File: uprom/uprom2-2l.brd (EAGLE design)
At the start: 40.6 x 25.4 mm, 7 parts, among them IC1 27C128P, IC2 74AC00D

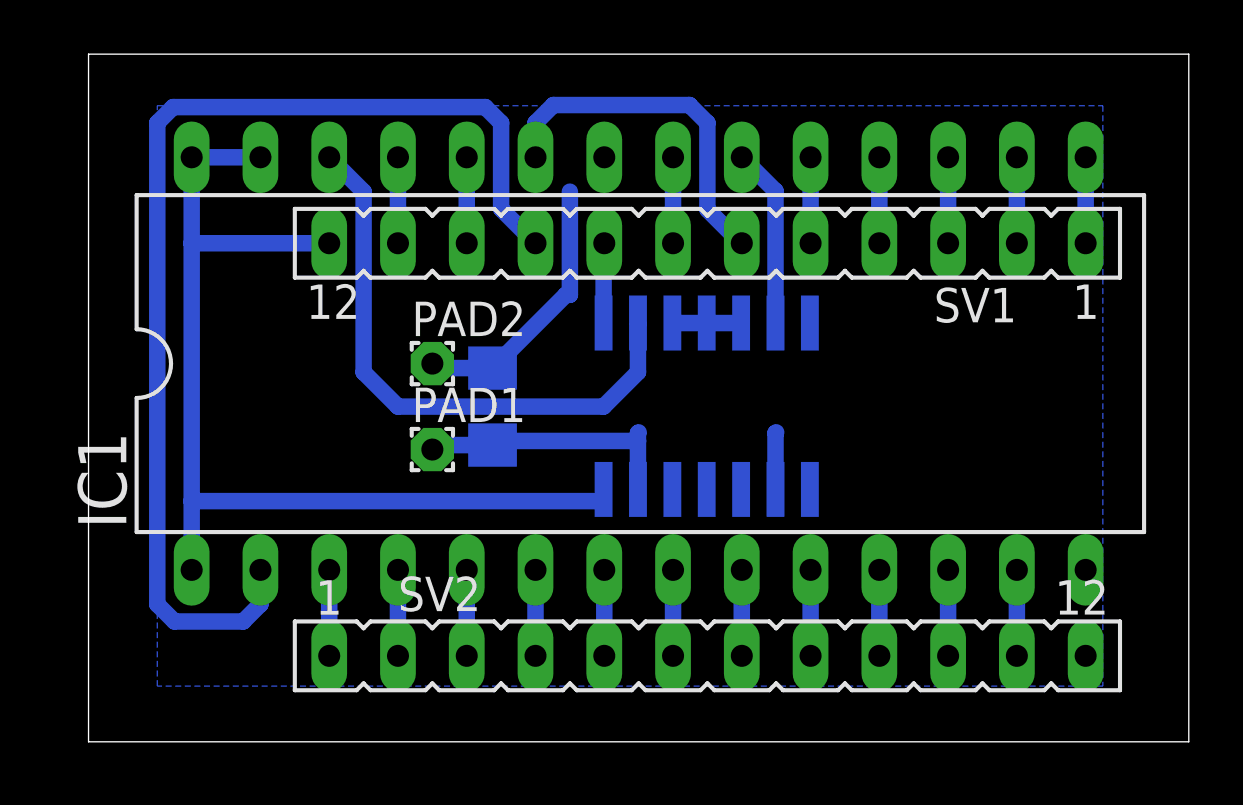
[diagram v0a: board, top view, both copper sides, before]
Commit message: final boards
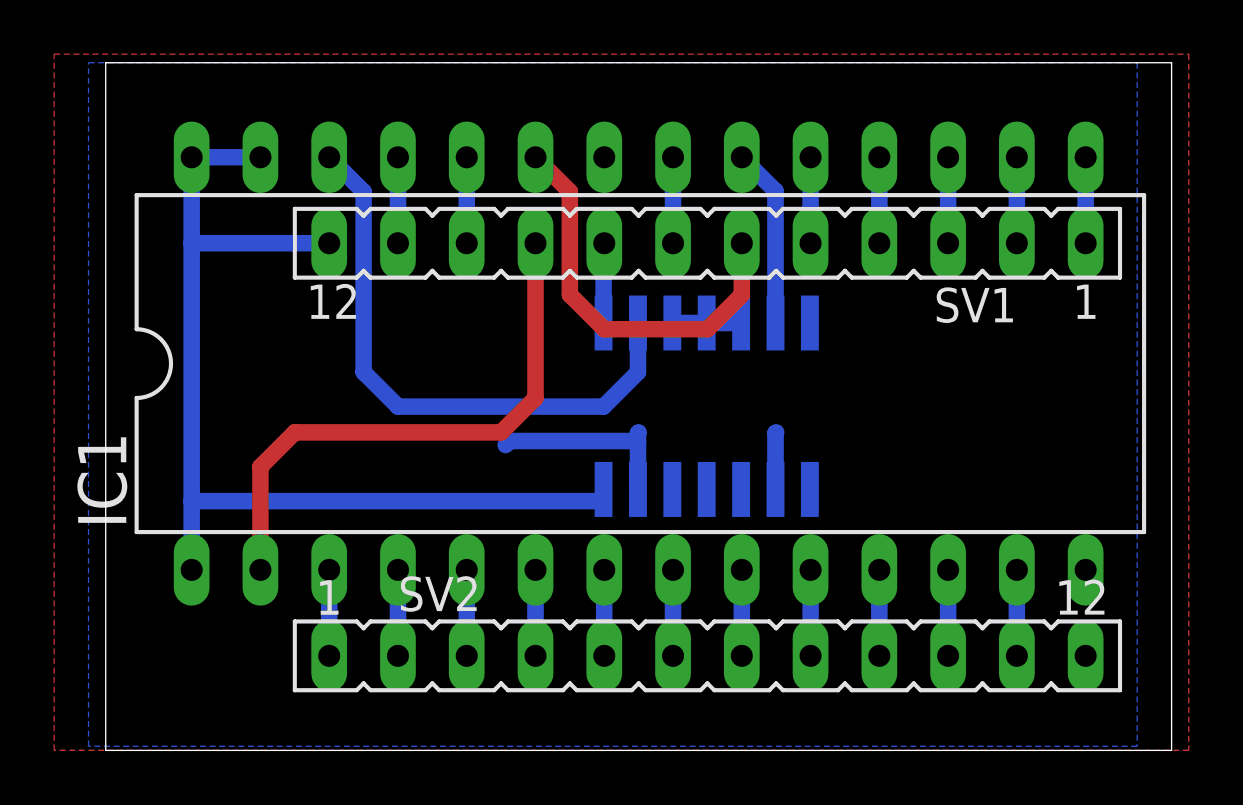
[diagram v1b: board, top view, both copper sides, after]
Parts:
- removed PAD1, PAD2: (no value), wirepad:1,6/0,8
- removed R1: (no value), rcl:R1206
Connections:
- net GND: no longer PAD1.1, PAD2.1, R1.1, R1.2
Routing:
- net A12: track 41.5 -> 20.7 mm
- net GND: track 22.0 -> 9.19 mm
- net A11: track 13.2 -> 14.9 mm
- added copper zone on layer 1, net GND
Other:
- board size 40.6 x 25.4 mm -> 39.4 x 25.4 mm
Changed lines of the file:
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@@
 <board>
 <plain>
-<wire x1="-62.23" y1="73.66" x2="-21.59" y2="73.66" width="0" layer="20"/>
-<wire x1="-21.59" y1="73.66" x2="-21.59" y2="99.06" width="0" layer="20"/>
-<wire x1="-21.59" y1="99.06" x2="-62.23" y2="99.06" width="0" layer="20"/>
-<wire x1="-62.23" y1="99.06" x2="-62.23" y2="73.66" width="0" layer="20"/>
+<wire x1="-61.595" y1="73.3425" x2="-22.225" y2="73.3425" width="0" layer="20"/>
+<wire x1="-22.225" y1="73.3425" x2="-22.225" y2="98.7425" width="0" layer="20"/>
+<wire x1="-22.225" y1="98.7425" x2="-61.595" y2="98.7425" width="0" layer="20"/>
+<wire x1="-61.595" y1="98.7425" x2="-61.595" y2="73.3425" width="0" layer="20"/>
 </plain>
 <attributes>
@@
 <attribute name="VALUE" x="-42.5704" y="86.8172" size="1.27" layer="28" ratio="10" rot="MR180"/>
 </element>
-<element name="R1" library="rcl" library_urn="urn:adsk.eagle:library:334" package="R1206" package3d_urn="urn:adsk.eagle:package:23540/2" value="" x="-47.3075" y="86.0425" smashed="yes" rot="MR270">
-<attribute name="NAME" x="-48.5775" y="87.3125" size="1.27" layer="26" rot="MR270"/>
-<attribute name="POPULARITY" value="41" x="-47.3075" y="86.0425" size="1.778" layer="28" rot="MR270" display="off"/>
-<attribute name="SPICEPREFIX" value="R" x="-47.3075" y="86.0425" size="1.778" layer="28" rot="MR270" display="off"/>
-<attribute name="VALUE" x="-44.7675" y="87.3125" size="1.27" layer="28" rot="MR270"/>
-</element>
-<element name="PAD1" library="wirepad" library_urn="urn:adsk.eagle:library:412" package="1,6/0,8" package3d_urn="urn:adsk.eagle:package:30830/1" value="" x="-49.53" y="84.455" smashed="yes">
-<attribute name="NAME" x="-50.292" y="85.471" size="1.27" layer="25" ratio="10"/>
-<attribute name="POPULARITY" value="15" x="-49.53" y="84.455" size="1.778" layer="27" display="off"/>
-<attribute name="VALUE" x="-49.53" y="85.055" size="0.0254" layer="27"/>
-</element>
-<element name="PAD2" library="wirepad" library_urn="urn:adsk.eagle:library:412" package="1,6/0,8" package3d_urn="urn:adsk.eagle:package:30830/1" value="" x="-49.53" y="87.63" smashed="yes">
-<attribute name="NAME" x="-50.292" y="88.646" size="1.27" layer="25" ratio="10"/>
-<attribute name="POPULARITY" value="15" x="-49.53" y="87.63" size="1.778" layer="27" display="off"/>
-<attribute name="VALUE" x="-49.53" y="88.23" size="0.0254" layer="27"/>
-</element>
 </elements>
 <signals>
@@
 <contactref element="IC1" pad="14"/>
 <contactref element="SV2" pad="12"/>
-<polygon width="0.508" layer="16" isolate="0.4064">
-<vertex x="-59.69" y="75.7174"/>
-<vertex x="-59.69" y="97.155"/>
-<vertex x="-24.765" y="97.155"/>
-<vertex x="-24.765" y="75.7174"/>
+<polygon width="0.508" layer="16" isolate="0.8128">
+<vertex x="-62.23" y="73.4949"/>
+<vertex x="-62.23" y="98.7425"/>
+<vertex x="-23.495" y="98.7425"/>
+<vertex x="-23.495" y="73.4949"/>
 </polygon>
 <contactref element="IC2" pad="7"/>
@@
 <wire x1="-36.8554" y1="85.0646" x2="-36.83" y2="85.09" width="0.6096" layer="16"/>
 <contactref element="IC1" pad="22"/>
-<contactref element="R1" pad="1"/>
-<contactref element="R1" pad="2"/>
-<wire x1="-47.3075" y1="84.6205" x2="-46.8245" y2="84.6205" width="0.6096" layer="16"/>
 <wire x1="-46.8245" y1="84.6205" x2="-46.6725" y2="84.7725" width="0.6096" layer="16"/>
 <wire x1="-46.6725" y1="84.7725" x2="-41.9354" y2="84.7725" width="0.6096" layer="16"/>
-<wire x1="-47.3075" y1="87.4645" x2="-44.602" y2="90.17" width="0.6096" layer="16"/>
-<wire x1="-44.602" y1="90.17" x2="-44.45" y2="90.17" width="0.6096" layer="16"/>
-<wire x1="-44.45" y1="90.17" x2="-44.45" y2="93.98" width="0.6096" layer="16"/>
-<contactref element="PAD1" pad="1"/>
-<contactref element="PAD2" pad="1"/>
-<wire x1="-47.3075" y1="87.4645" x2="-49.3645" y2="87.4645" width="0.6096" layer="16"/>
-<wire x1="-49.3645" y1="87.4645" x2="-49.53" y2="87.63" width="0.6096" layer="16"/>
-<wire x1="-47.3075" y1="84.6205" x2="-49.3645" y2="84.6205" width="0.6096" layer="16"/>
-<wire x1="-49.3645" y1="84.6205" x2="-49.53" y2="84.455" width="0.6096" layer="16"/>
-<wire x1="-47.3075" y1="84.6205" x2="-47.3075" y2="87.4645" width="0" layer="19" extent="16-16"/>
+<polygon width="0.6096" layer="1" isolate="0.4064">
+<vertex x="-63.5" y="99.06"/>
+<vertex x="-21.59" y="99.06"/>
+<vertex x="-21.59" y="73.3425"/>
+<vertex x="-63.5" y="73.3425"/>
+</polygon>
 </signal>
 <signal name="!CS">
@@
 <contactref element="IC1" pad="2"/>
 <contactref element="SV1" pad="9"/>
-<wire x1="-45.72" y1="92.075" x2="-46.99" y2="93.345" width="0.6096" layer="16"/>
-<wire x1="-46.99" y1="93.345" x2="-46.99" y2="96.52" width="0.6096" layer="16"/>
-<wire x1="-46.99" y1="96.52" x2="-47.5742" y2="97.1042" width="0.6096" layer="16"/>
-<wire x1="-59.1058" y1="97.1042" x2="-59.69" y2="96.52" width="0.6096" layer="16"/>
-<wire x1="-59.69" y1="96.52" x2="-59.69" y2="78.74" width="0.6096" layer="16"/>
-<wire x1="-59.69" y1="78.74" x2="-59.055" y2="78.105" width="0.6096" layer="16"/>
-<wire x1="-59.055" y1="78.105" x2="-56.515" y2="78.105" width="0.6096" layer="16"/>
-<wire x1="-56.515" y1="78.105" x2="-55.88" y2="78.74" width="0.6096" layer="16"/>
-<wire x1="-55.88" y1="78.74" x2="-55.88" y2="80.01" width="0.6096" layer="16"/>
-<wire x1="-47.5742" y1="97.1042" x2="-59.1058" y2="97.1042" width="0.6096" layer="16"/>
+<wire x1="-55.88" y1="80.01" x2="-55.88" y2="83.82" width="0.6096" layer="1"/>
+<wire x1="-55.88" y1="83.82" x2="-54.61" y2="85.09" width="0.6096" layer="1"/>
+<wire x1="-54.61" y1="85.09" x2="-46.99" y2="85.09" width="0.6096" layer="1"/>
+<wire x1="-46.99" y1="85.09" x2="-45.72" y2="86.36" width="0.6096" layer="1"/>
+<wire x1="-45.72" y1="86.36" x2="-45.72" y2="92.075" width="0.6096" layer="1"/>
 </signal>
 <signal name="A7">
@@
 <contactref element="SV1" pad="6"/>
 <contactref element="IC1" pad="23"/>
-<wire x1="-45.72" y1="95.25" x2="-45.72" y2="96.52" width="0.6096" layer="16"/>
-<wire x1="-45.72" y1="96.52" x2="-45.0596" y2="97.1804" width="0.6096" layer="16"/>
-<wire x1="-45.0596" y1="97.1804" x2="-40.0304" y2="97.1804" width="0.6096" layer="16"/>
-<wire x1="-40.0304" y1="97.1804" x2="-39.37" y2="96.52" width="0.6096" layer="16"/>
-<wire x1="-39.37" y1="96.52" x2="-39.37" y2="93.3196" width="0.6096" layer="16"/>
-<wire x1="-39.37" y1="93.3196" x2="-38.1254" y2="92.075" width="0.6096" layer="16"/>
-<wire x1="-38.1254" y1="92.075" x2="-38.1" y2="92.075" width="0.6096" layer="16"/>
+<wire x1="-45.72" y1="95.25" x2="-44.45" y2="93.98" width="0.6096" layer="1"/>
+<wire x1="-44.45" y1="93.98" x2="-44.45" y2="90.17" width="0.6096" layer="1"/>
+<wire x1="-44.45" y1="90.17" x2="-43.18" y2="88.9" width="0.6096" layer="1"/>
+<wire x1="-43.18" y1="88.9" x2="-39.37" y2="88.9" width="0.6096" layer="1"/>
+<wire x1="-39.37" y1="88.9" x2="-38.1" y2="90.17" width="0.6096" layer="1"/>
+<wire x1="-38.1" y1="90.17" x2="-38.1" y2="92.075" width="0.6096" layer="1"/>
 </signal>
 <signal name="D0">
